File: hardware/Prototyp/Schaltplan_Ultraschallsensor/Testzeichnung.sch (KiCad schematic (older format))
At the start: 14 parts, among them U3 LMR62014X

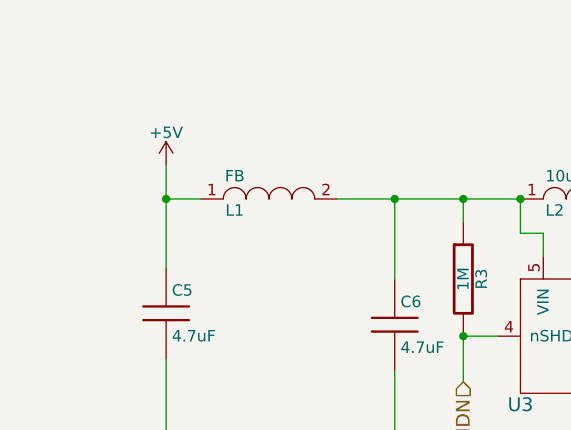
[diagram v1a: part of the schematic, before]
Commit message: Layout
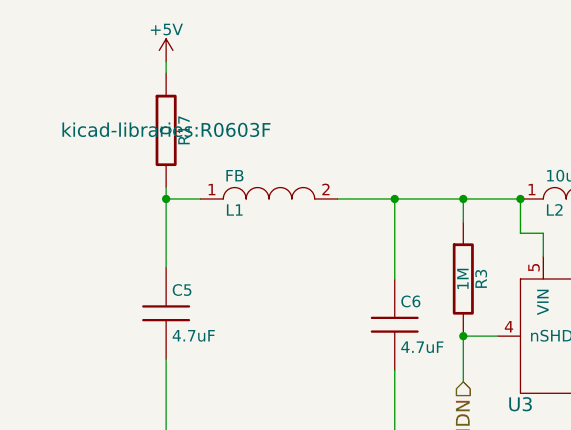
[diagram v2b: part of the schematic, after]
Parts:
- added R17: 0, kicad-libraries:R0603F, symbol R
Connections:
- net +5V: now also R17.1; no longer C5.1, L1.1
- new net: C5.1, L1.1, R17.2
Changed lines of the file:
@@
 Connection ~ 9100 1400
 Connection ~ 6100 2000
-Wire Wire Line
-	4800 1250 4800 1700
 $Comp
 L +5V #PWR031
 U 1 1 5A793374
-P 4800 1250
-F 0 "#PWR031" H 4800 1100 50  0001 C CNN
-F 1 "+5V" H 4800 1390 50  0000 C CNN
-F 2 "" H 4800 1250 50  0001 C CNN
-F 3 "" H 4800 1250 50  0001 C CNN
-	1    4800 1250
+P 4800 800
+F 0 "#PWR031" H 4800 650 50  0001 C CNN
+F 1 "+5V" H 4800 940 50  0000 C CNN
+F 2 "" H 4800 800 50  0001 C CNN
+F 3 "" H 4800 800 50  0001 C CNN
+	1    4800 800
 	1    0    0    -1
 $EndComp
+$Comp
+L R R17
+U 1 1 5A795820
+P 4800 1100
+F 0 "R17" V 4880 1100 50  0000 C CNN
+F 1 "0" V 4800 1100 50  0000 C CNN
+F 2 "kicad-libraries:R0603F" H 4800 1100 60  0000 C CNN
+F 3 "" H 4800 1100 60  0000 C CNN
+	1    4800 1100
+	1    0    0    -1
+$EndComp
+Wire Wire Line
+	4800 1350 4800 1700
+Wire Wire Line
+	4800 850  4800 800
 $EndSCHEMATC
